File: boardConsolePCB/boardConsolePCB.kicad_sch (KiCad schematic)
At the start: 132 parts, among them J1 to HV cable, J2 SMA F, J3 PROG, J4 BUTTONS, J5 PWR, J6 FUEL/TRIM, J7 PRG_UART, Q1 BC548, Q2 IRML0030TR, Q3 IRML0030TR, U1 NE555P, U2 AZ1117-3.3, U3 STM32G071RBTx, U5 L76-L, U6 AZ1117-5.0, U7 ABC016002C34-FHA-R-01, U8 TXS0108EPW, U9 AT24C04C, X1 Bart's Design, Y2 16M

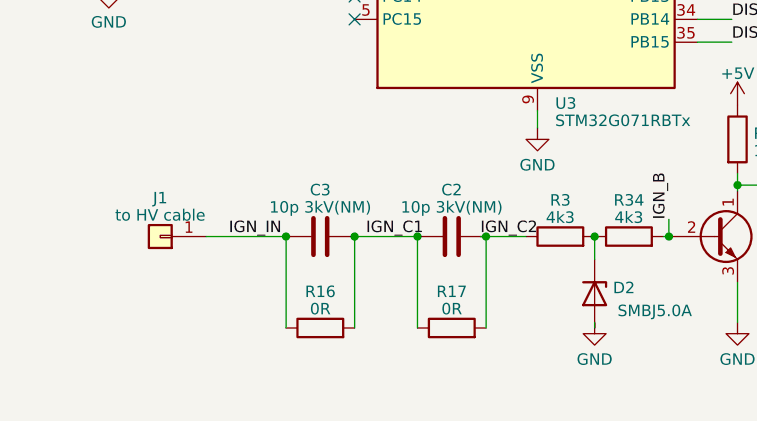
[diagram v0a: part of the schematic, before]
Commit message: add GDT
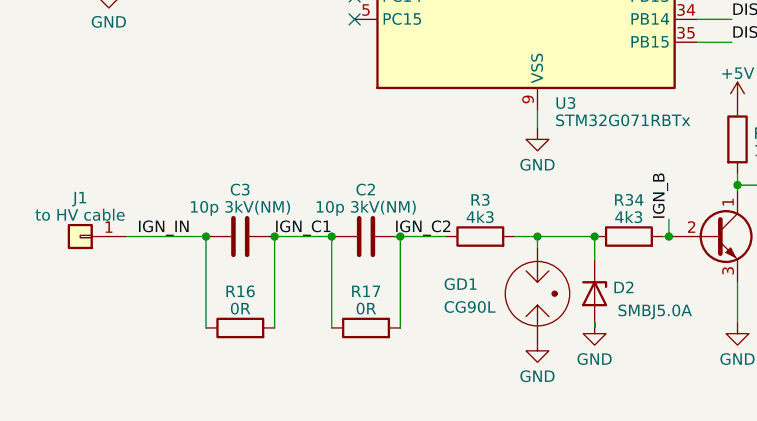
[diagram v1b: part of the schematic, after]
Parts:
- added GD1: CG90L, boardConsoleLib:CG90L, symbol Device:GDT_2Pin
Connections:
- net GND: now also GD1.1
- net at D2.1 (K), R3.2, R34.1: now also GD1.3
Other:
- moved on the sheet: C2, C3, J1, R16, R17, R3
